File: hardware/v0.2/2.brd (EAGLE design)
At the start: 54.9 x 27.5 mm, 36 parts, among them IC1 STM32F10XCXT6, U1 ADXL345"

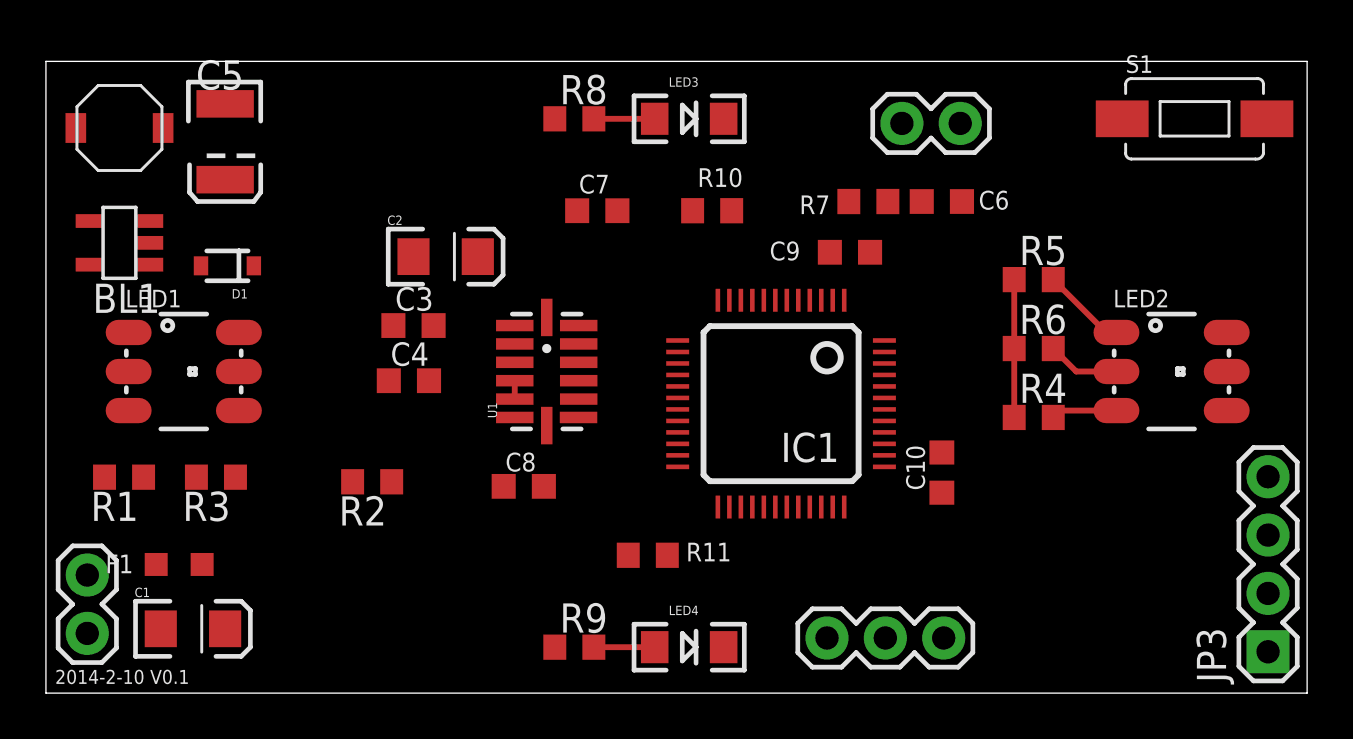
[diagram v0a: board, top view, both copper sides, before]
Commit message: update PCB design
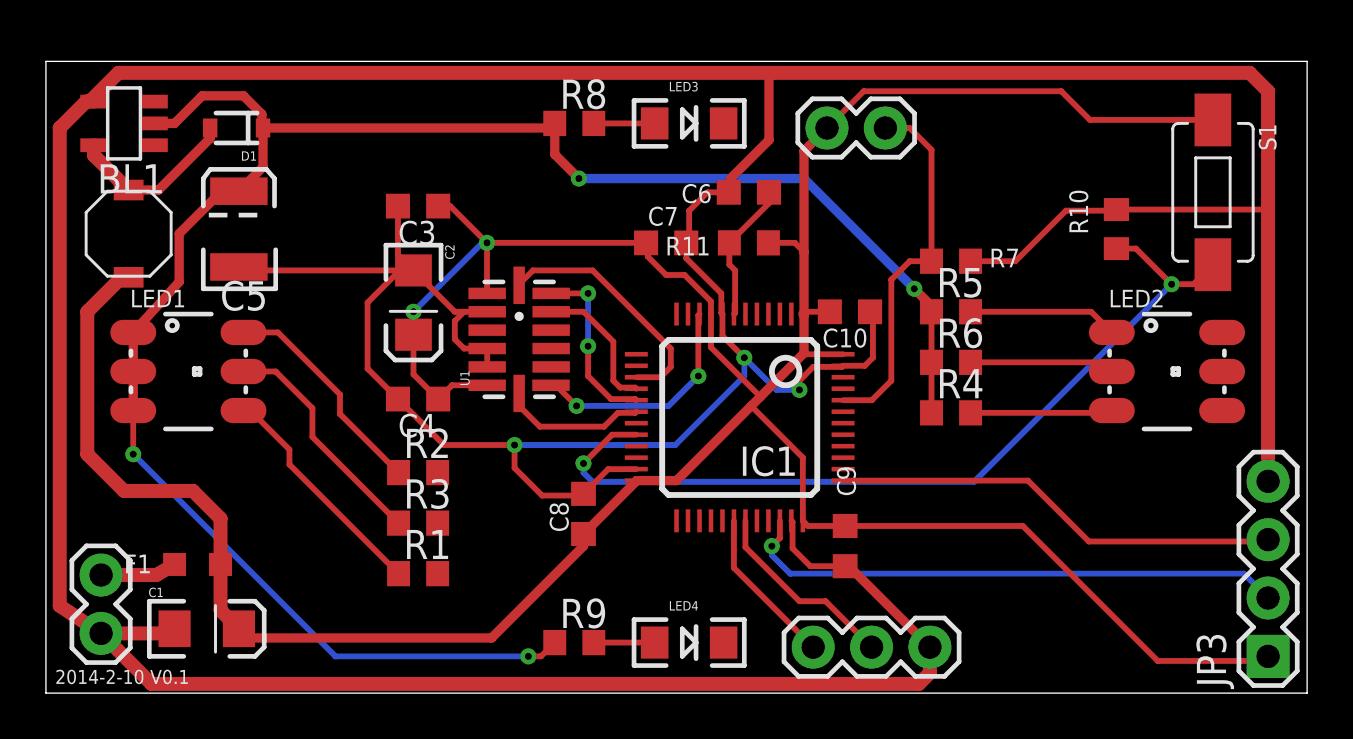
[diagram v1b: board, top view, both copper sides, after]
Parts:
- moved R10 17.6 mm to (46.6, 20.2), turned to 90 degrees
- moved R11 14.3 mm to (30.6, 19.6), turned to 180 degrees
- moved R1 13.5 mm to (16.2, 5.20), turned to 0 degrees
- moved C9 12.8 mm to (34.8, 6.40), turned to 270 degrees
- moved R3 9.02 mm to (16.2, 7.40), turned to 0 degrees
- moved C6 8.41 mm to (30.6, 21.8), turned to 180 degrees
- moved C10 8.06 mm to (35.0, 16.6), turned to 0 degrees
- moved D1 6.01 mm to (8.30, 24.6)
- moved JP4 5.80 mm to (34.0, 24.6), turned to 0 degrees
- moved BL1 5.20 mm to (3.40, 24.8)
- moved C3 5.20 mm to (16.2, 21.2), turned to 180 degrees
- moved L1 4.62 mm to (3.60, 20.0), turned to 90 degrees
- moved R7 4.44 mm to (39.4, 18.8), turned to 180 degrees
- moved R5 3.86 mm to (39.4, 16.6)
- moved C5 3.85 mm to (8.40, 20.2), turned to 90 degrees
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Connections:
- removed net LED1_B: LED1.4
- removed net LED1_G: LED1.6
- removed net LED1_R: LED1.5
- removed net XL345_INT: IC1.13, U1.8
- net 3.3V: now also LED1.1, LED1.2, LED1.3; no longer R1.1, R2.1, R3.1
- net N$6: now also LED1.4, R1.1; no longer LED1.3, R1.2
- net N$7: now also LED1.6, R2.1; no longer LED1.1, R2.2
- net N$8: now also LED1.5, R3.1; no longer LED1.2, R3.2
- net WAKEUP: now also U1.8; no longer U1.9
- net XL345_CS: now also IC1.18; no longer IC1.14
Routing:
- net GND: track 0.80 -> 234.1 mm, vias 0 -> 3
- net 2.8V: track 0.00 -> 145.1 mm, vias 0 -> 2
- net 3.3V: track 6.00 -> 83.2 mm, vias 0 -> 4
- net N$2: track 0.00 -> 37.7 mm, vias 0 -> 2
- net SWDIO: track 0.00 -> 24.0 mm, vias 0 -> 1
- net SWCLK: track 0.00 -> 19.6 mm
- net BOOT0: track 0.00 -> 16.2 mm
- net XL345_SCK: track 0.00 -> 10.8 mm
- net N$8: track 0.00 -> 10.2 mm
- net N$6: track 0.00 -> 10.1 mm
- net WAKEUP: track 0.00 -> 10.0 mm, vias 0 -> 2
- net N$7: track 0.00 -> 9.77 mm
- net USART1_RX: track 0.00 -> 8.44 mm
- net XL345_MOSI: track 0.00 -> 7.74 mm, vias 0 -> 2
- net N$12: track 0.00 -> 7.51 mm
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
